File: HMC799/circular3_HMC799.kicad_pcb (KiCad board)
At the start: 2 copper layers, 25 x 25 mm, 31 parts, among them J101 Conn_Coaxial, J102 Conn_01x02, U101 LT3042xMSE, U103 HMC799LP3E, U104 BUF602xDBV

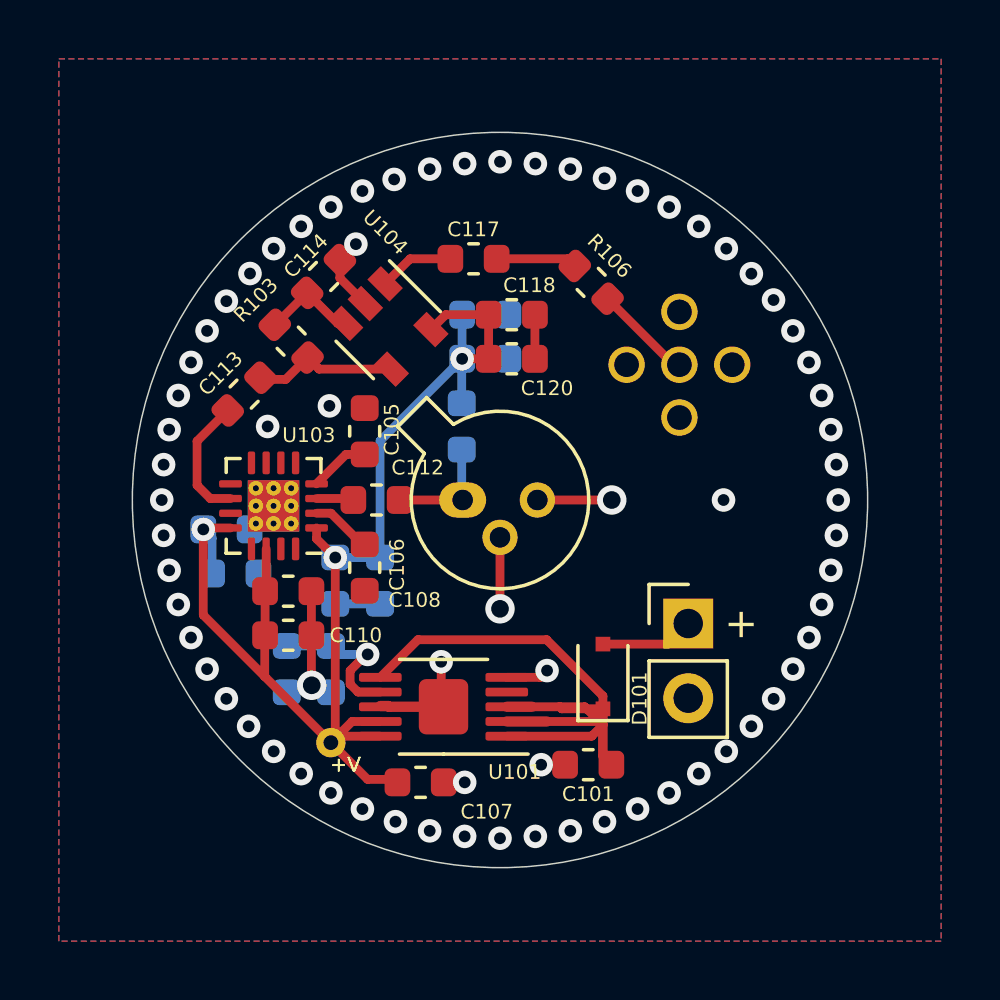
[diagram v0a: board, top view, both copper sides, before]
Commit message: 0402 caps
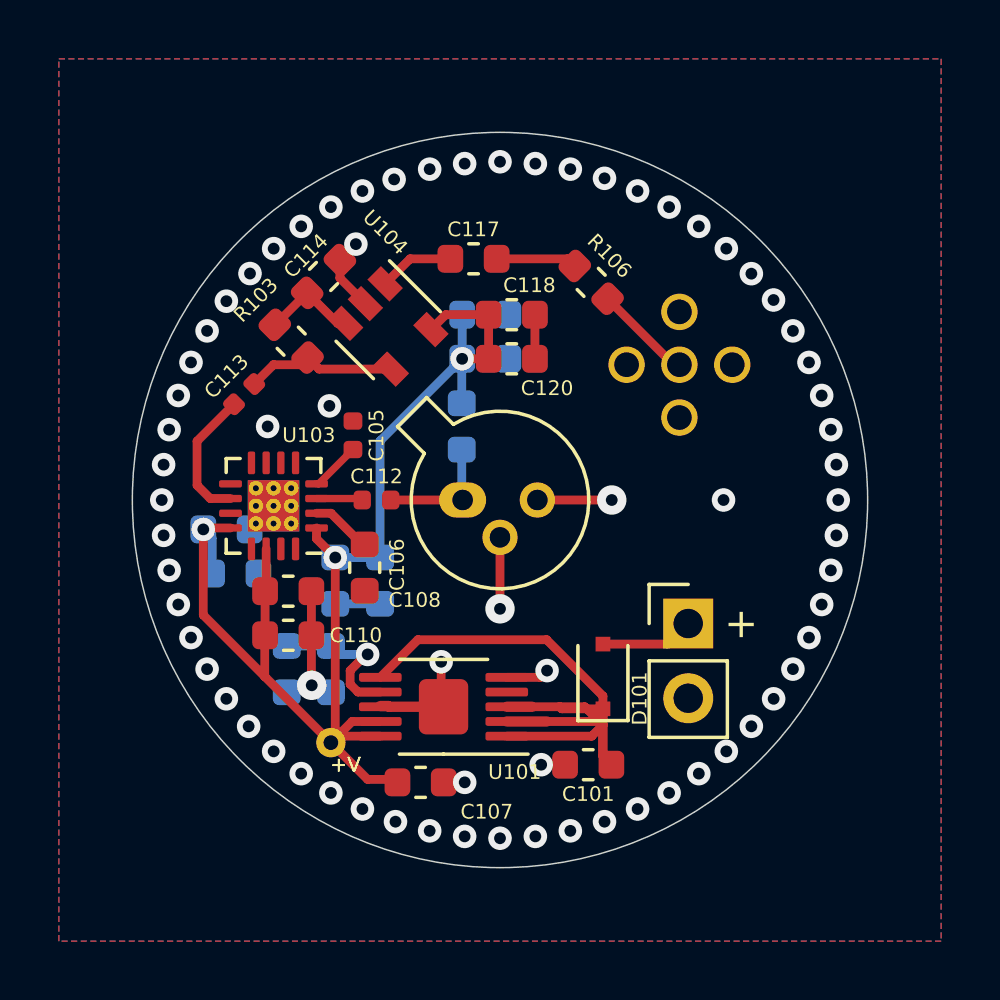
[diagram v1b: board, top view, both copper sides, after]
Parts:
- C105, C112, C113: footprint Capacitor_SMD:C_0603_1608Metric -> Capacitor_SMD:C_0402_1005Metric
- moved C105 0.42 mm to (145.0, 97.8)
